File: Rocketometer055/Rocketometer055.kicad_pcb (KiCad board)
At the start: 2 copper layers, 55.9 x 22.9 mm, 65 parts, among them J001 USB_MICROB, J301 JST 2mm, J701 Micro_SD_Card_Det_Hirose_DM3AT, Q050 PMOS, U101 BME280, U201 3.3V, U301 MCP73831, U401 LPC2148, U501 FGPMMOPA6H, U501 MPU9250, U601 BNO085, U901 ADXL375, X511 uFL, Y401 12MHz, Y601 32kiHz

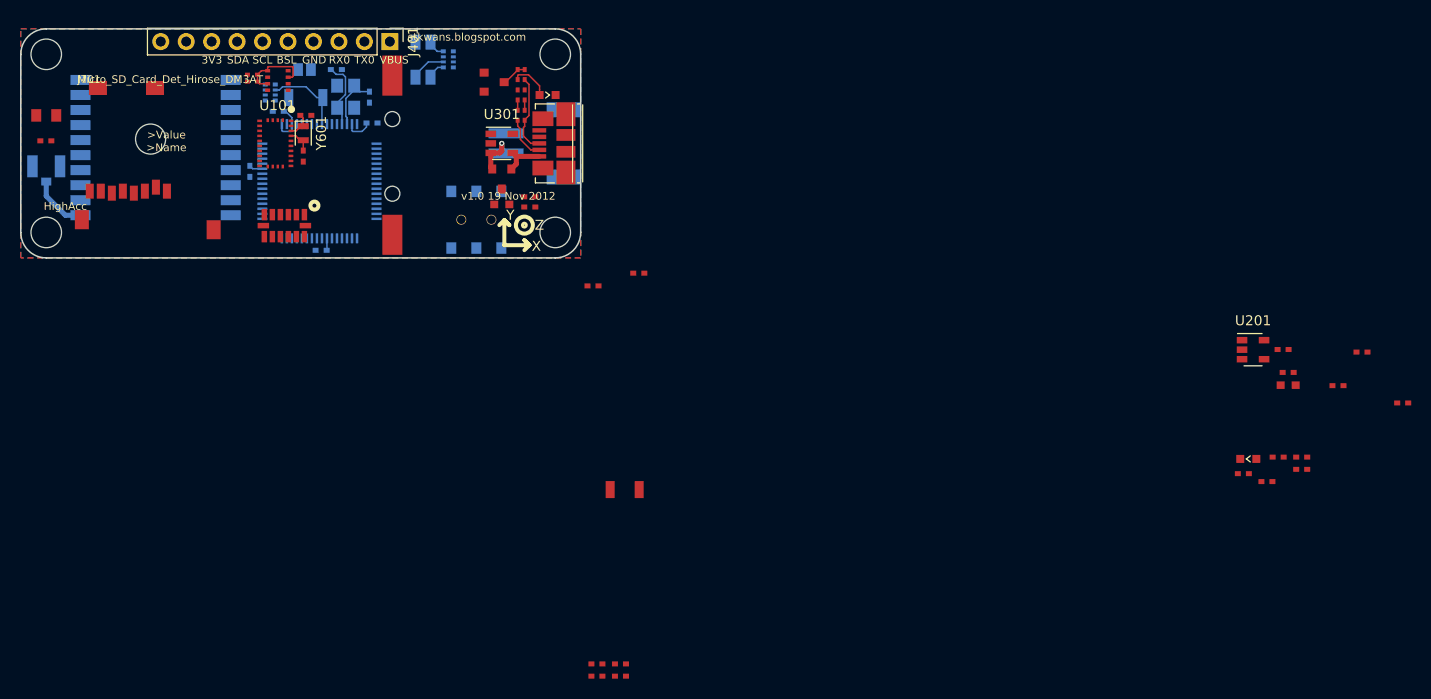
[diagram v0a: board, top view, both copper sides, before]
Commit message: More work on Rocketometer055
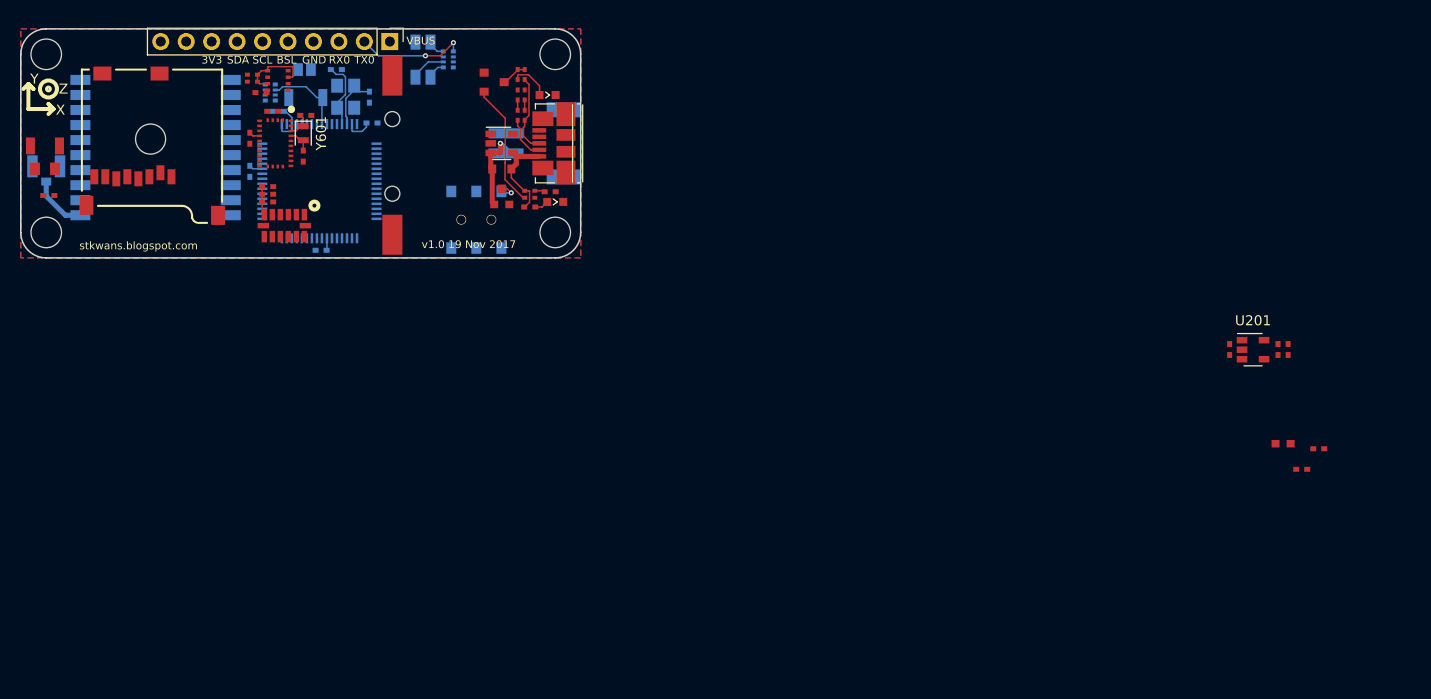
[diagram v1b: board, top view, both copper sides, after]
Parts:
- removed C010: 1uF, KwanSystems:SMD_0402
- removed C020, C030: 22pF, KwanSystems:SMD_0402
- removed R010: 10k, KwanSystems:SMD_0402
- D401: footprint KwanSystems:HSMF-C118 -> HSMF-C118
- J701: footprint KwanSystems:MICROSD-SOCKET-PP -> MICROSD-SOCKET-PP
- R051: footprint KwanSystems:SMD_0402 -> KwanSystems:R_Array_Convex_2x0402
- moved R011 79.5 mm to (179.8, 95.0), turned to 180 degrees
- moved R051 79.0 mm to (177.8, 95.2)
- moved D301 73.8 mm to (180.3, 96.0), turned to 180 degrees
- moved C503 67.3 mm to (129.4, 90.4)
- moved C901 66.1 mm to (151.0, 85.1)
- moved R906 60.2 mm to (151.6, 94.5), turned to 180 degrees
- moved C906 58.6 mm to (151.6, 95.2)
- moved C905 57.6 mm to (151.6, 96.0)
- moved U501 49.4 mm to (127.8, 86.7)
- moved C603 39.9 mm to (152.1, 87.0)
- moved C609 37.3 mm to (149.9, 89.7), turned to 90 degrees
- moved C215 13.2 mm to (253.5, 110.7), turned to 270 degrees
- moved C214 10.7 mm to (252.5, 110.7), turned to 90 degrees
- moved R302 8.21 mm to (256.5, 120.7)
- moved C302 5.86 mm to (253.0, 120.1)
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- renumbered C914 to C905, C916 to C906, R914 to R906
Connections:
- net /TX0/PWMR renamed /TX0(PWMR)
- net Net-(C914-Pad1) renamed /HighAcc/VS
- J401 pad 7: (no net) -> /SDA(BSL)
- J401 pad 8: (no net) -> /SCL
- R051 pad 1: /USB_SOFTCONNECT -> /VBUS
- R401 pad 1: /SDA/BSL -> /SDA(BSL)
- U101 pad 3: /SDA/BSL -> /SDA(BSL)
- U401 pad 41: /SDA/BSL -> /SDA(BSL)
- U601 pad 20: /SDA/BSL -> /SDA(BSL)
- U901 pad 13: /SDA/BSL -> /SDA(BSL)
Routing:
- net VCC: track 16.7 -> 29.1 mm
- net /TX0(PWMR): track 0.00 -> 10.9 mm, vias 0 -> 2
- net /VBUS: track 4.82 -> 9.96 mm
- net /VLIPO: track 5.47 -> 9.09 mm
- net /HighAcc/VS: track 0.00 -> 2.89 mm
- net /VIN: track 0.00 -> 2.14 mm, vias 0 -> 1
- net /STAT+: track 0.00 -> 1.40 mm
- net /BNO055/CAP: track 0.00 -> 1.11 mm
- net /USB_ON: track 0.00 -> 1.02 mm
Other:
- board text added: "v1.0 19 Nov 2017"
- board text removed: "HighAcc"
- board text removed: "Reset"
- board text removed: "St Kwan's Home for"
- board text removed: "a division of"
- board text removed: "the Terminally ADD"
- board text removed: "v1.0 19 Nov 2012"
